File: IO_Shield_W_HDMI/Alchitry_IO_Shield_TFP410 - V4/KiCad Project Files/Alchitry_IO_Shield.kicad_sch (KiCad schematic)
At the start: 1 part, among them U0 boardmezzanine_new

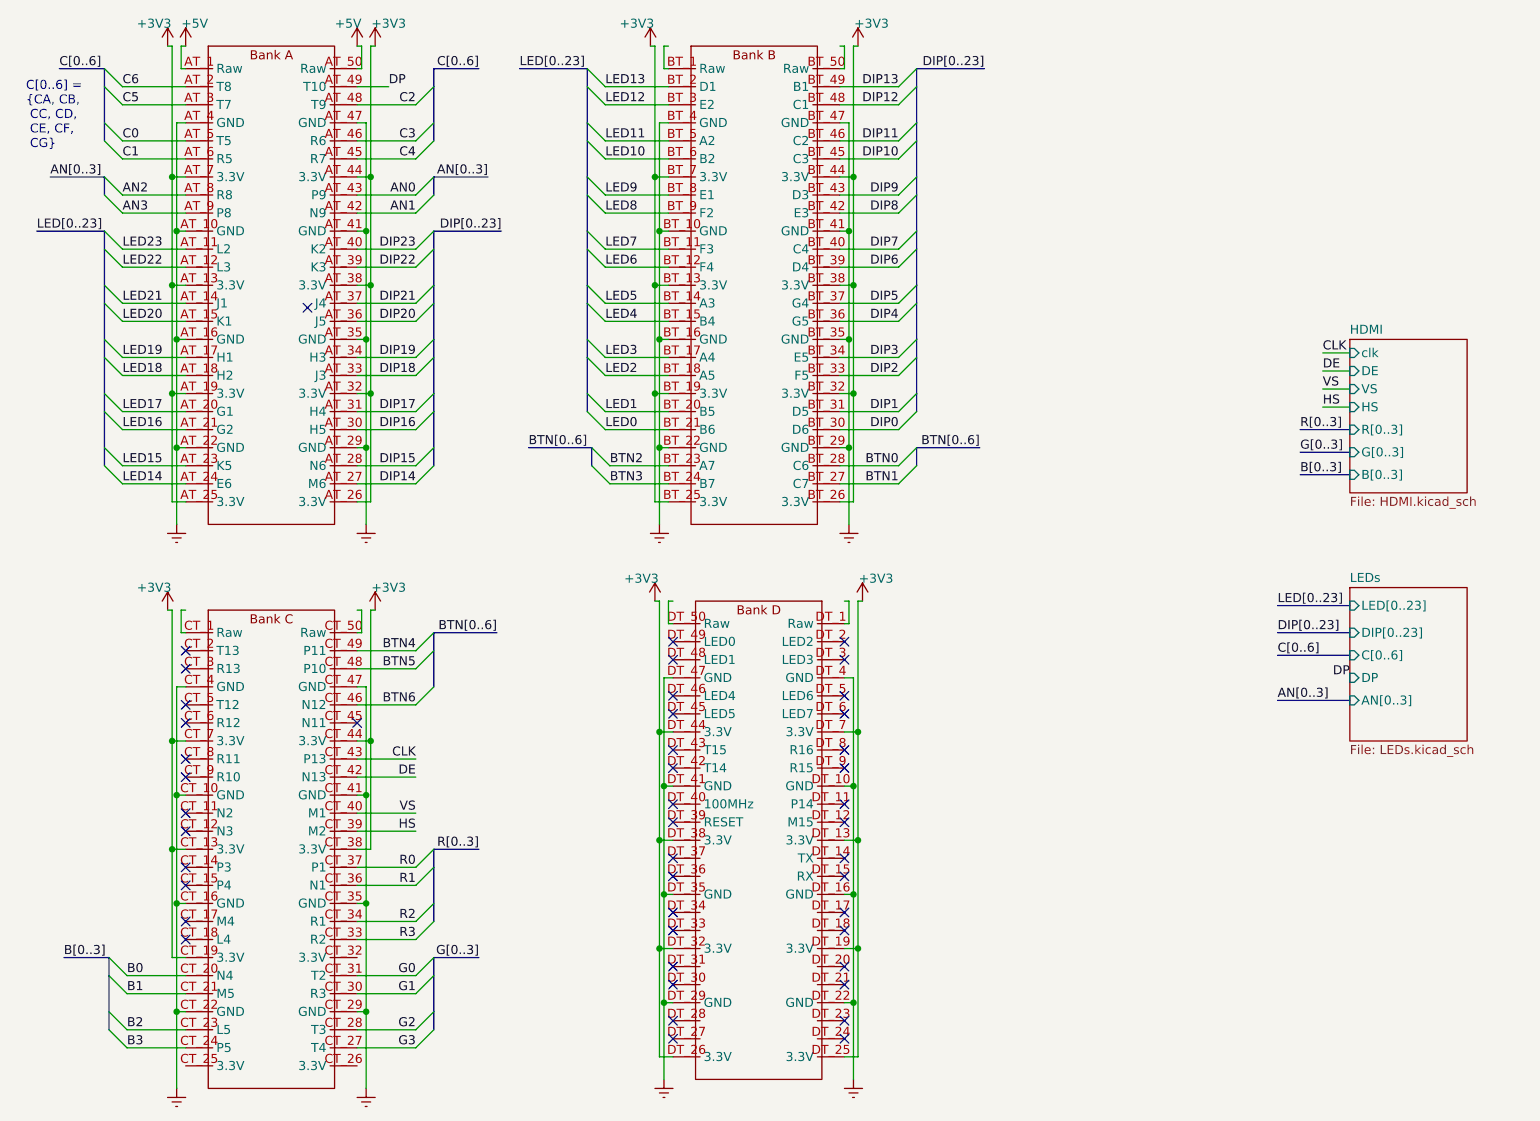
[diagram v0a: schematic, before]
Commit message: minor changes
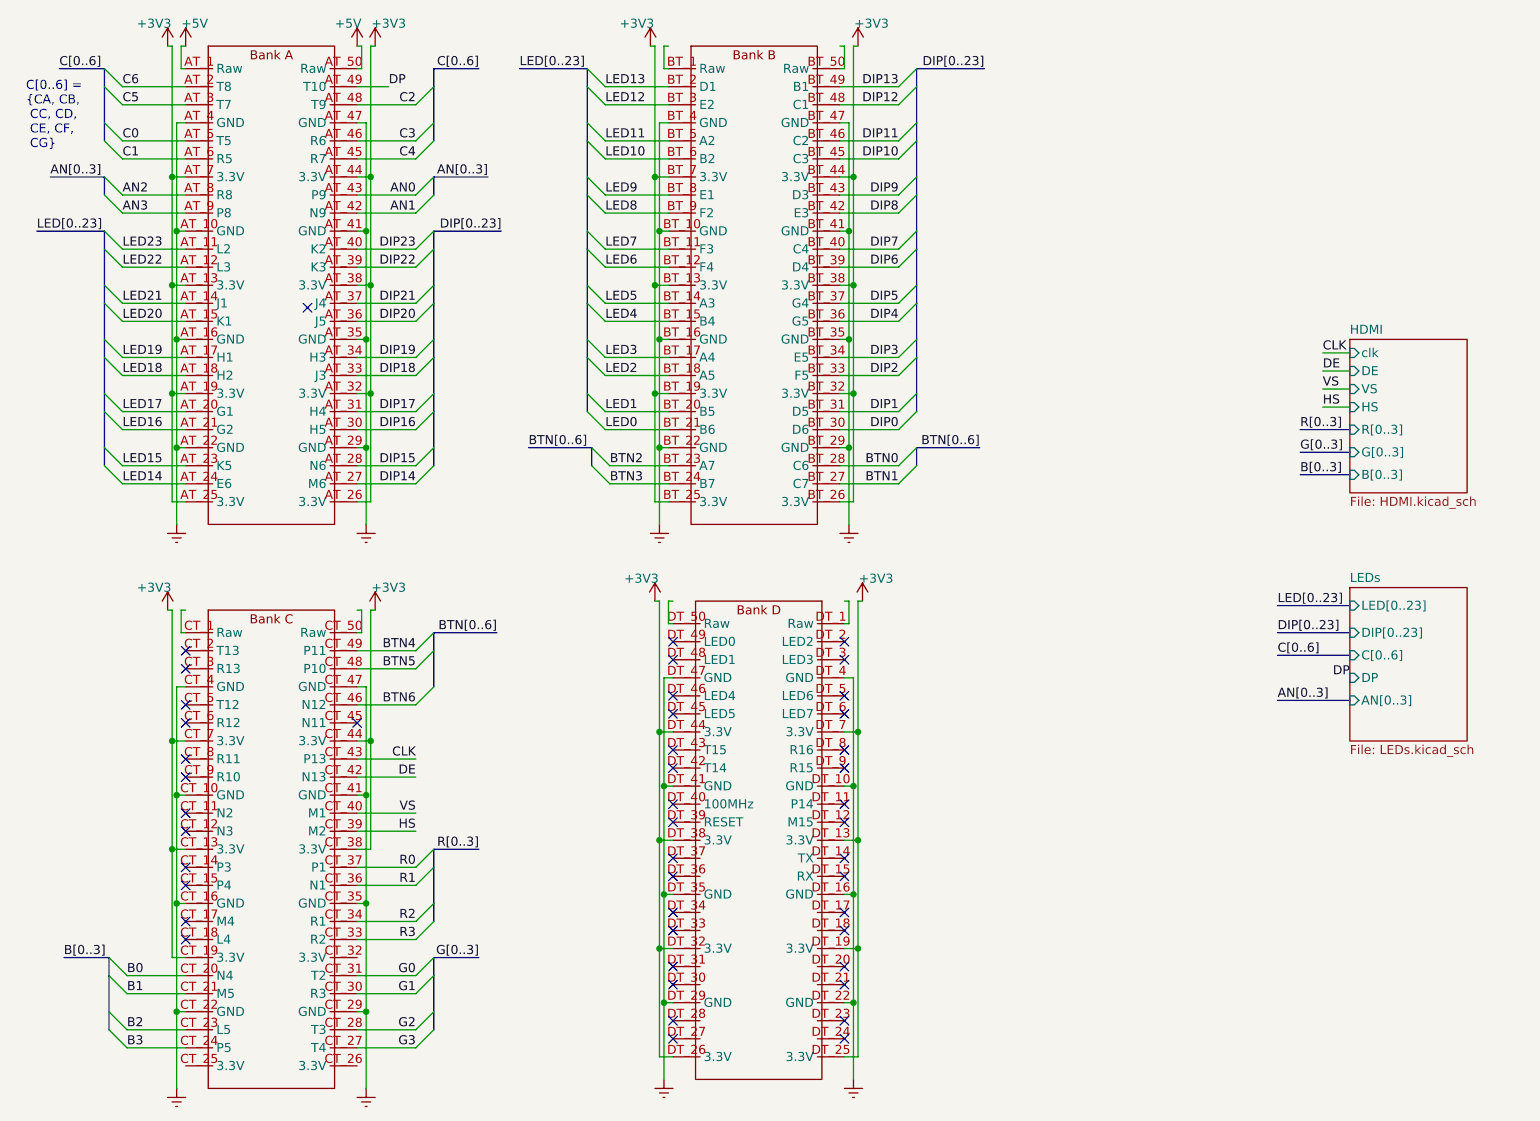
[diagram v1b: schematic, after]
